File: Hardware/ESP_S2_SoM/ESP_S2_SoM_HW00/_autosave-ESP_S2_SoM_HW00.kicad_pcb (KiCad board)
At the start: 6 copper layers, 20 x 20 mm, 54 parts, among them J1 DF40C-60DP-0.4V(51), J2 Bare PCB USB C, SW401 SW_Push, SW402 SW_Push, U201 BQ24075RGTR, U301 MIC5528-3.3YMT-T5, U401 ESP32-S2FH4, Y601 Crystal_GND24_Small

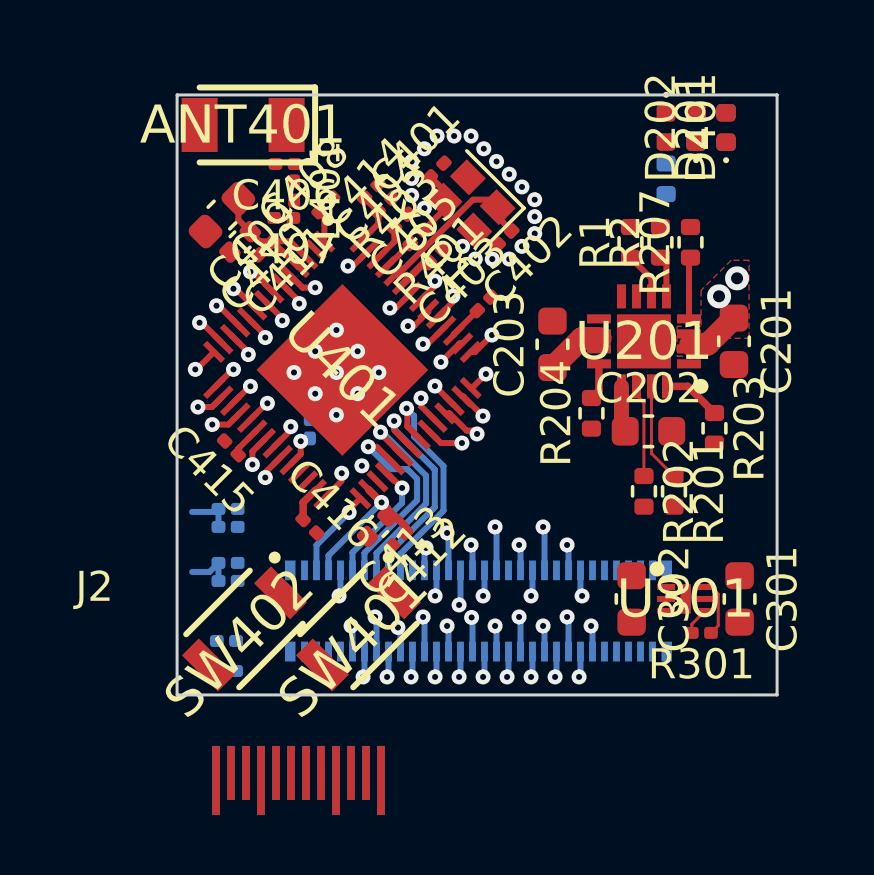
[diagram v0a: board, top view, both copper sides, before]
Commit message: Continue work on routing
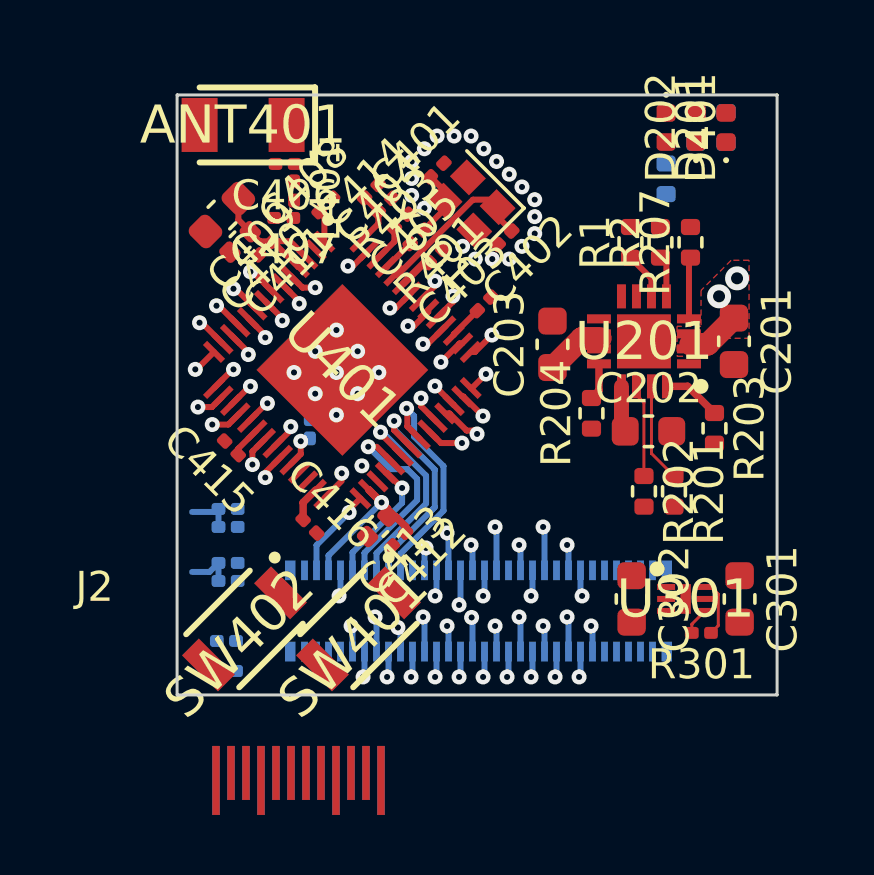
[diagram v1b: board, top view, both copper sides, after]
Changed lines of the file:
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@@
   (segment (start 138.646853 108.353147) (end 138.6 108.4) (width 0.2) (layer "B.Cu") (net 27))
   (segment (start 138.646853 107.555) (end 138.646853 108.353147) (width 0.2) (layer "B.Cu") (net 27))
+  (segment (start 133.23467 100.174831) (end 133.23467 99.865896) (width 0.2) (layer "F.Cu") (net 28))
   (segment (start 133.807857 100.748018) (end 133.23467 100.174831) (width 0.2) (layer "F.Cu") (net 28))
   (via (at 133.23467 99.865896) (size 0.5) (drill 0.2) (layers "F.Cu" "B.Cu") (net 28))
@@
       88d7b2f9-51ff-4618-85b4-a46eb3845e83
       8972854a-11ad-4be9-82df-055edb75dd6e
-      89e8b359-9524-4d40-99a1-6c09b65607d2
       8b863f6f-576f-4519-8ab6-a60e47461337
       8bb94d68-46c0-4bf3-9581-a56377ac94e9
